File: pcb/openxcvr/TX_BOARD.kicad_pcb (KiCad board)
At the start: 2 copper layers, 99.1 x 63.5 mm, 68 parts, among them J1 Power Amplifier, J2 RADIO_CONNECTOR, J3 Antenna, J4 12V_IN, K1 G5V-2, K2 G5V-2, K3 G5V-2, K5 G5V-2, Q1 BS170, Q2 BS170, Q3 BS170, Q4 BS170, U1 LM7805_TO220

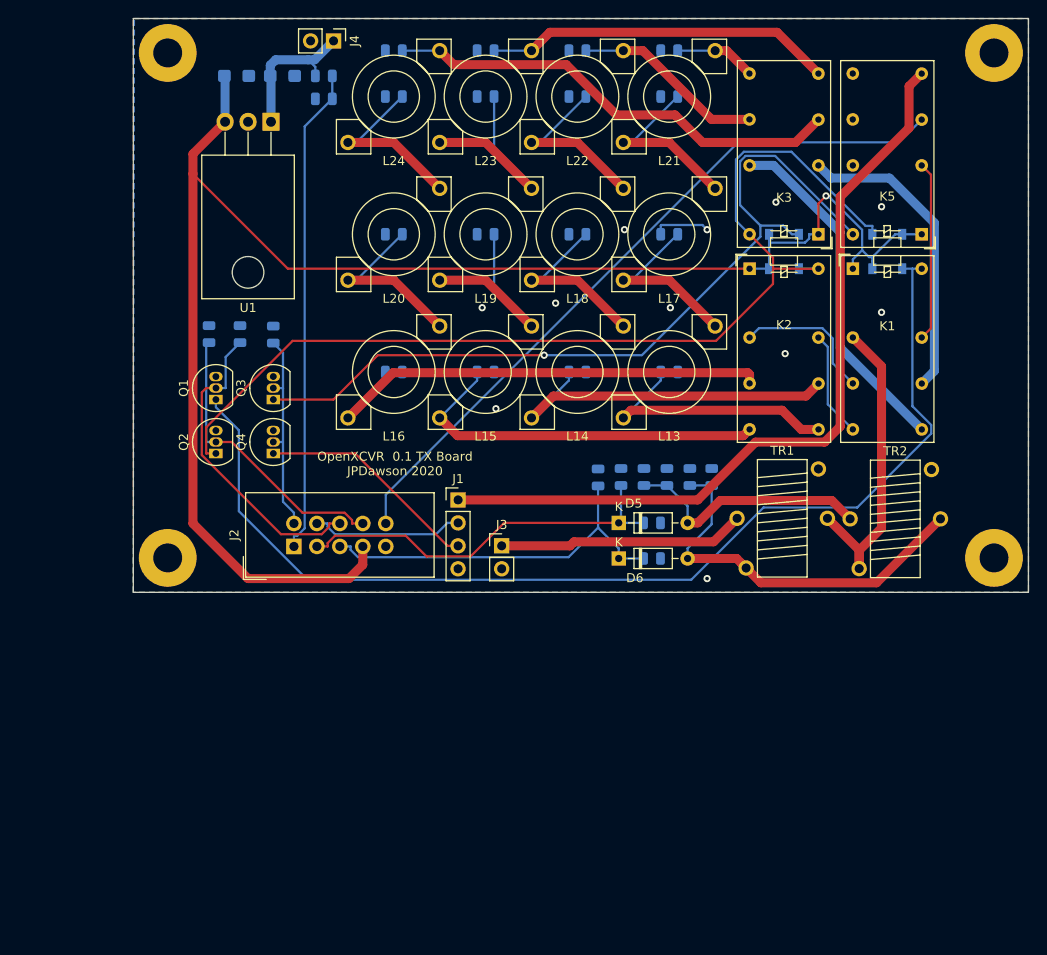
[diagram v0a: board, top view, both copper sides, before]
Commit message: update rev0.2 PCB
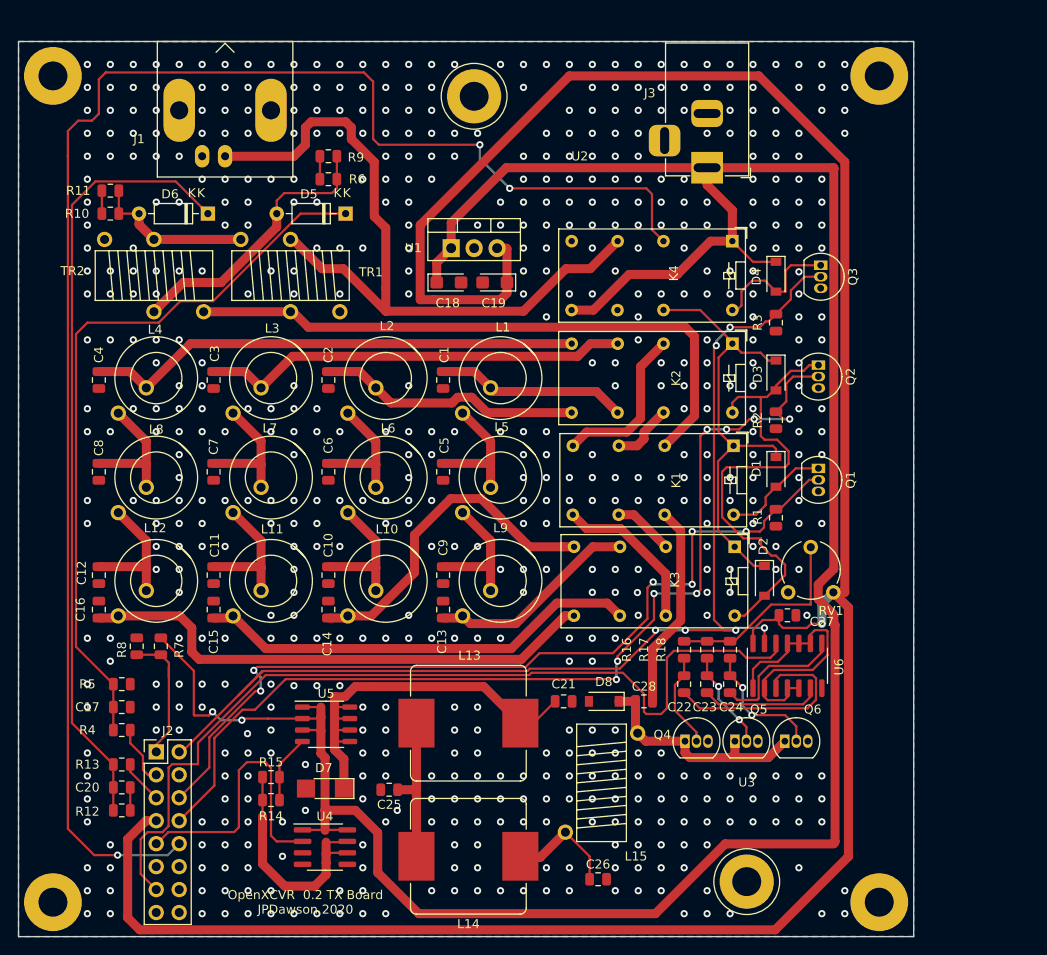
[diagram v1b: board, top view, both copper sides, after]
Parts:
- removed C55, C67: 470p, Capacitor_SMD:C_0805_2012Metric
- removed C56, C68: 270p, Capacitor_SMD:C_0805_2012Metric
- removed C57, C69: 180p, Capacitor_SMD:C_0805_2012Metric
- removed C58, C70: 56p, Capacitor_SMD:C_0805_2012Metric
- removed C59, C63: 1.2n, Capacitor_SMD:C_0805_2012Metric
- removed C60, C64: 680p, Capacitor_SMD:C_0805_2012Metric
- removed C61, C65: 390p, Capacitor_SMD:C_0805_2012Metric
- removed C62, C66: 150p, Capacitor_SMD:C_0805_2012Metric
- removed J4: 12V_IN, Connector_PinHeader_2.54mm:PinHeader_1x02_P2.54mm_Vertical
- removed K5: G5V-2, Relay_THT:Relay_DPDT_Omron_G5V-2
- removed L17: 3.012u, openxcvr:FT37-INDUCTOR
- removed L18: 1.698u, openxcvr:FT37-INDUCTOR
- removed L19: 904n, openxcvr:FT37-INDUCTOR
- removed L20: 382n, openxcvr:FT37-INDUCTOR
- removed L21: 2.434u, openxcvr:FT37-INDUCTOR
- removed L22: 1.380u, openxcvr:FT37-INDUCTOR
- removed L23: 773n, openxcvr:FT37-INDUCTOR
- removed L24: 303n, openxcvr:FT37-INDUCTOR
- removed the R7 at (158.1, 101.5)
- added C10: 390p, Capacitor_SMD:C_0805_2012Metric, F.Cu at (123.2, 112.4)
- added C11: 680p, Capacitor_SMD:C_0805_2012Metric, F.Cu at (110.5, 112.4)
- added C12: 1.2n, Capacitor_SMD:C_0805_2012Metric, F.Cu at (97.8, 112.4)
- added C13: 56p, Capacitor_SMD:C_0805_2012Metric, F.Cu at (135.9, 116.2)
- added C14: 180p, Capacitor_SMD:C_0805_2012Metric, F.Cu at (123.2, 116.2)
- added C15: 270p, Capacitor_SMD:C_0805_2012Metric, F.Cu at (110.5, 116.2)
- added C16: 470p, Capacitor_SMD:C_0805_2012Metric, F.Cu at (97.8, 116.2)
- added C17: 100n, Capacitor_SMD:C_0805_2012Metric, F.Cu at (100.3, 127.0)
- added C2: 180p, Capacitor_SMD:C_0805_2012Metric, F.Cu at (123.2, 90.8)
- added C21: 68n, Capacitor_SMD:C_0805_2012Metric, F.Cu at (149.2, 126.4)
- added C22: 100n, Capacitor_SMD:C_0805_2012Metric, F.Cu at (162.6, 124.5)
- added C23: 100n, Capacitor_SMD:C_0805_2012Metric, F.Cu at (165.1, 124.5)
- added C24: 100n, Capacitor_SMD:C_0805_2012Metric, F.Cu at (167.6, 124.5)
- added C25: 220n, Capacitor_SMD:C_0805_2012Metric, F.Cu at (129.9, 136.1)
- added C26: 68n, Capacitor_SMD:C_0805_2012Metric, F.Cu at (153.0, 146.1)
- added C27: C, Capacitor_SMD:C_0805_2012Metric, F.Cu at (174.0, 116.8)
- added C28: 100n, Capacitor_SMD:C_0805_2012Metric, F.Cu at (158.1, 126.4)
- added C3: 270p, Capacitor_SMD:C_0805_2012Metric, F.Cu at (110.5, 90.8)
- added C4: 470p, Capacitor_SMD:C_0805_2012Metric, F.Cu at (97.8, 90.8)
- added C5: 150p, Capacitor_SMD:C_0805_2012Metric, F.Cu at (135.9, 101.0)
- added C6: 390p, Capacitor_SMD:C_0805_2012Metric, F.Cu at (123.2, 101.0)
- added C7: 680p, Capacitor_SMD:C_0805_2012Metric, F.Cu at (110.5, 101.0)
- added C8: 1.2n, Capacitor_SMD:C_0805_2012Metric, F.Cu at (97.8, 101.0)
- added C9: 150p, Capacitor_SMD:C_0805_2012Metric, F.Cu at (135.9, 112.4)
- added D7: D_Schottky, openxcvr:D_SOD-106, F.Cu at (122.8, 136.0)
- added D8: 51v, Diode_SMD:D_SOD-123, F.Cu at (153.7, 126.4)
- added K4: G5V-2, Relay_THT:Relay_DPDT_Omron_G5V-2, F.Cu at (167.9, 75.4)
- added L10: 773n, openxcvr:FT37-INDUCTOR, F.Cu at (129.5, 105.4)
- added L11: 1.380u, openxcvr:FT37-INDUCTOR, F.Cu at (116.8, 105.4)
- added L12: 2.434u, openxcvr:FT37-INDUCTOR, F.Cu at (104.1, 105.4)
- added L13: 100u, openxcvr:L_SMT_INDUCTOR, F.Cu at (138.7, 128.8)
- added L14: 100u, openxcvr:L_SMT_INDUCTOR, F.Cu at (138.7, 143.5)
- added L15: L, openxcvr:FT50-43 INDUCTOR, F.Cu at (153.4, 143.4)
- added L5: 382n, openxcvr:FT37-INDUCTOR, F.Cu at (142.2, 94.0)
- added L6: 904n, openxcvr:FT37-INDUCTOR, F.Cu at (129.5, 94.0)
- added L7: 1.698u, openxcvr:FT37-INDUCTOR, F.Cu at (116.8, 94.0)
- added L8: 3.012u, openxcvr:FT37-INDUCTOR, F.Cu at (104.1, 94.0)
- added L9: 303n, openxcvr:FT37-INDUCTOR, F.Cu at (142.2, 105.4)
- added Q5: BS170, Package_TO_SOT_THT:TO-92_Inline, F.Cu at (168.2, 130.8)
- added Q6: BS170, Package_TO_SOT_THT:TO-92_Inline, F.Cu at (173.7, 130.8)
- added R13: 10k, Resistor_SMD:R_0805_2012Metric, F.Cu at (100.3, 133.3)
- added R14: 10, Resistor_SMD:R_0805_2012Metric, F.Cu at (116.8, 137.3)
- added R15: 10, Resistor_SMD:R_0805_2012Metric, F.Cu at (116.8, 134.7)
- added R16: 4k7, Resistor_SMD:R_0805_2012Metric, F.Cu at (162.6, 120.7)
- added R17: 4k7, Resistor_SMD:R_0805_2012Metric, F.Cu at (165.1, 120.7)
- added R18: 4k7, Resistor_SMD:R_0805_2012Metric, F.Cu at (167.6, 120.7)
- added R6: 100, Resistor_SMD:R_0805_2012Metric, F.Cu at (123.2, 68.6)
- added R9: 100, Resistor_SMD:R_0805_2012Metric, F.Cu at (123.2, 66.0)
- added RV1: 10k, Potentiometer_THT:Potentiometer_Piher_PT-6-V_Vertical, F.Cu at (179.1, 114.3)
- added U2: to220heatsink, openxcvr:to220 heatsink, F.Cu at (139.3, 72.4)
- added U3: to220heatsink, openxcvr:to220 heatsink, F.Cu at (169.5, 133.3)
- added U4: MCP1406, Package_SO:SOIC-8_3.9x4.9mm_P1.27mm, F.Cu at (122.8, 142.5)
- added U5: DMC3056LSS, Package_SO:SOP-8_3.9x4.9mm_P1.27mm, F.Cu at (122.9, 128.9)
- added U6: 74AC00, Package_SO:SOIC-14_3.9x8.7mm_P1.27mm, F.Cu at (174.0, 122.4)
- C1: value 100n -> 56p; moved to F.Cu
- C18: renamed from C2; moved to F.Cu
- C19: renamed from C3; moved to F.Cu
- C20: renamed from C4; moved to F.Cu
- D1, D2, D3, D4, R1, R2, R3: moved to F.Cu
- J1: value Power Amplifier -> Conn_Coaxial; footprint Connector_PinHeader_2.54mm:PinHeader_1x04_P2.54mm_Vertical -> Connector_Coaxial:BNC_Amphenol_B6252HB-NPP3G-50_Horizontal
- J2: value RADIO_CONNECTOR -> Conn_02x08_Odd_Even; footprint Connector_IDC:IDC-Header_2x05_P2.54mm_Vertical -> Connector_PinHeader_2.54mm:PinHeader_2x08_P2.54mm_Vertical
- J3: value Antenna -> Barrel_Jack_Switch; footprint Connector_PinHeader_2.54mm:PinHeader_1x02_P2.54mm_Vertical -> Connector_BarrelJack:BarrelJack_Horizontal
- R10: renamed from R8; moved to F.Cu
- R11: renamed from R9; moved to F.Cu
- R12: renamed from R11; moved to F.Cu
- R4: value 100 -> 10k; moved to F.Cu
- R5: renamed from R10; moved to F.Cu
- R7: renamed from R5; moved to F.Cu
- R8: renamed from R6; moved to F.Cu
- U1: footprint Package_TO_SOT_THT:TO-220-3_Horizontal_TabDown -> Package_TO_SOT_THT:TO-220-3_Vertical
- moved TR2 92.0 mm to (95.9, 79.2), turned to 90 degrees
- moved R11 73.7 mm to (99.1, 69.8), turned to 180 degrees
- moved R10 70.4 mm to (99.1, 72.4), turned to 180 degrees
- moved Q2 67.4 mm to (177.4, 89.2), turned to -90 degrees
- moved Q1 67.1 mm to (177.4, 100.6), turned to -90 degrees
- moved R4 66.5 mm to (100.3, 129.5), turned to 180 degrees
- moved R7 65.6 mm to (104.6, 120.3), turned to -90 degrees
- moved R12 64.3 mm to (100.3, 138.4), turned to 0 degrees
- moved R8 64.0 mm to (102.0, 120.3), turned to 90 degrees
- moved C20 63.9 mm to (100.3, 135.9)
- moved R2 63.5 mm to (172.7, 95.2), turned to -90 degrees
- moved R1 62.7 mm to (172.7, 106.0), turned to -90 degrees
- moved Q3 62.4 mm to (177.7, 78.1), turned to -90 degrees
- moved R5 59.8 mm to (100.3, 124.5), turned to 0 degrees
- moved D6 59.4 mm to (109.9, 72.4), turned to 180 degrees
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- renumbered L16 to L1, L15 to L2, L14 to L3, L13 to L4
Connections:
- net LPF_SWR renamed SWR_IN
- C1 pad 1: FWD_PWR -> LPF_BAND_0_A
- C18 pad 1: Net-(C2-Pad1) -> +12V
- C20 pad 1: REV_PWR -> Net-(C20-Pad1)
- D1 pad 1: +5V -> LPF_ENABLE
- D2 pad 1: +5V -> LPF_ENABLE
- D3 pad 1: +5V -> LPF_ENABLE
- D3 pad 2: Net-(D3-Pad2) -> Net-(D2-Pad2)
- D4 pad 1: +5V -> +12V
- D4 pad 2: Net-(D2-Pad2) -> Net-(D4-Pad2)
- D5 pad 1: FWD_PWR -> Net-(C17-Pad1)
- D6 pad 1: REV_PWR -> Net-(C20-Pad1)
- J1 pad 1: PA_IN -> ANTENNA
- J1 pad 2: RF_IN -> GND
- J2 pad 4: RF_IN -> BAND_2
- J2 pad 9: GND -> RF_ENVELOPE
- J3 pad 1: ANTENNA -> +12V
- K1 pad 1: +5V -> LPF_ENABLE
- K1 pad 13: LPF_TXRX -> PA_OUT
- K2 pad 1: +5V -> LPF_ENABLE
- K2 pad 11: LPF_BAND_2_A -> LPF_BAND_0_A
- K2 pad 13: Net-(K1-Pad8) -> Net-(K1-Pad6)
- K2 pad 4: Net-(K1-Pad6) -> Net-(K1-Pad8)
- K2 pad 6: LPF_BAND_0_A -> LPF_BAND_2_A
- K2 pad 8: LPF_BAND_1_A -> LPF_BAND_3_A
- K2 pad 9: LPF_BAND_3_A -> LPF_BAND_1_A
- K3 pad 1: +5V -> LPF_ENABLE
- Q3 pad 1: Net-(D3-Pad2) -> Net-(D4-Pad2)
- Q4 pad 1: TX_N -> Net-(C28-Pad1)
- Q4 pad 2: TX_ENABLE -> Net-(C22-Pad2)
- R12 pad 1: REV_PWR -> Net-(C20-Pad1)
- R4 pad 1: Net-(D5-Pad2) -> FWD_PWR
- R4 pad 2: GND -> Net-(C17-Pad1)
- R5 pad 1: FWD_PWR -> Net-(C17-Pad1)
- R7 pad 1: Net-(C2-Pad1) -> +12V
- U1 pad 1: Net-(C2-Pad1) -> +12V
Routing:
- net +12V: track 0.00 -> 279.2 mm, vias 0 -> 2
- net Net-(D1-Pad2): track 121.1 -> 12.0 mm
- net TX_ENABLE: track 23.1 -> 126.7 mm, vias 0 -> 6
- net LO_I: track 0.00 -> 100.9 mm
- net RF_OUT: track 79.7 -> 176.9 mm, vias 0 -> 3
- net +5V: track 177.2 -> 272.3 mm
- net Net-(D3-Pad2): track 91.7 -> 0.00 mm, vias 1 -> 0
- net PA_IN: track 88.4 -> 0.00 mm
- net Net-(C20-Pad1): track 0.00 -> 86.5 mm
- net Net-(C17-Pad1): track 0.00 -> 80.9 mm
- net BAND_0: track 32.4 -> 111.5 mm, vias 0 -> 8
- net Net-(D2-Pad2): track 115.7 -> 52.8 mm
- net BAND_1: track 35.1 -> 95.7 mm, vias 0 -> 6
- net ANTENNA: track 27.3 -> 81.3 mm
- net LPF_ENABLE: track 0.00 -> 49.8 mm
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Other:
- board size 99.1 x 63.5 mm -> 99.1 x 99.1 mm
- board text added: "OpenXCVR 0.2 TX Board JPDawson 2020"
- board text removed: "OpenXCVR 0.1 TX Board JPDawson 2020"
